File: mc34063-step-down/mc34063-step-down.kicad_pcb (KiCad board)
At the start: 2 copper layers, 82 x 52 mm, 104 parts, among them J1 Vin, J2 Vout, U1 MC34063AD, U2 220uH

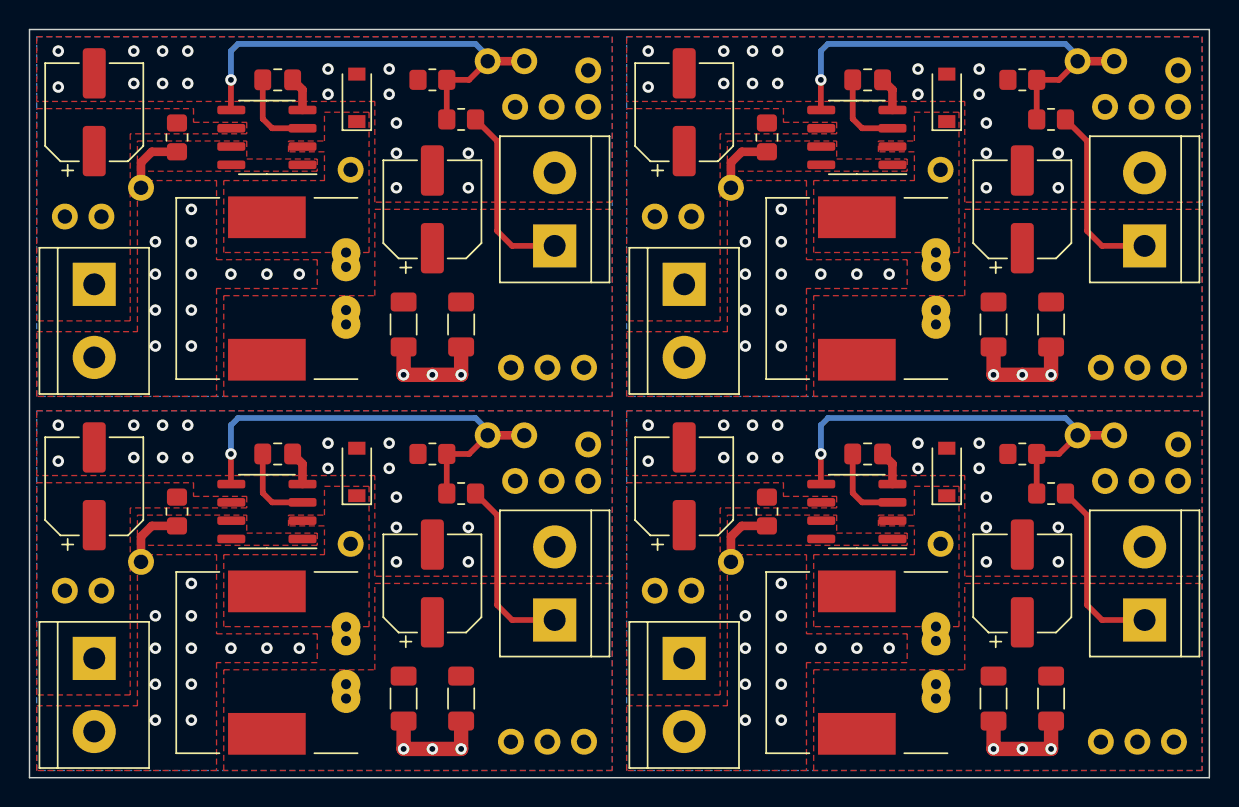
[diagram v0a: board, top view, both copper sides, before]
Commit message: released dev board
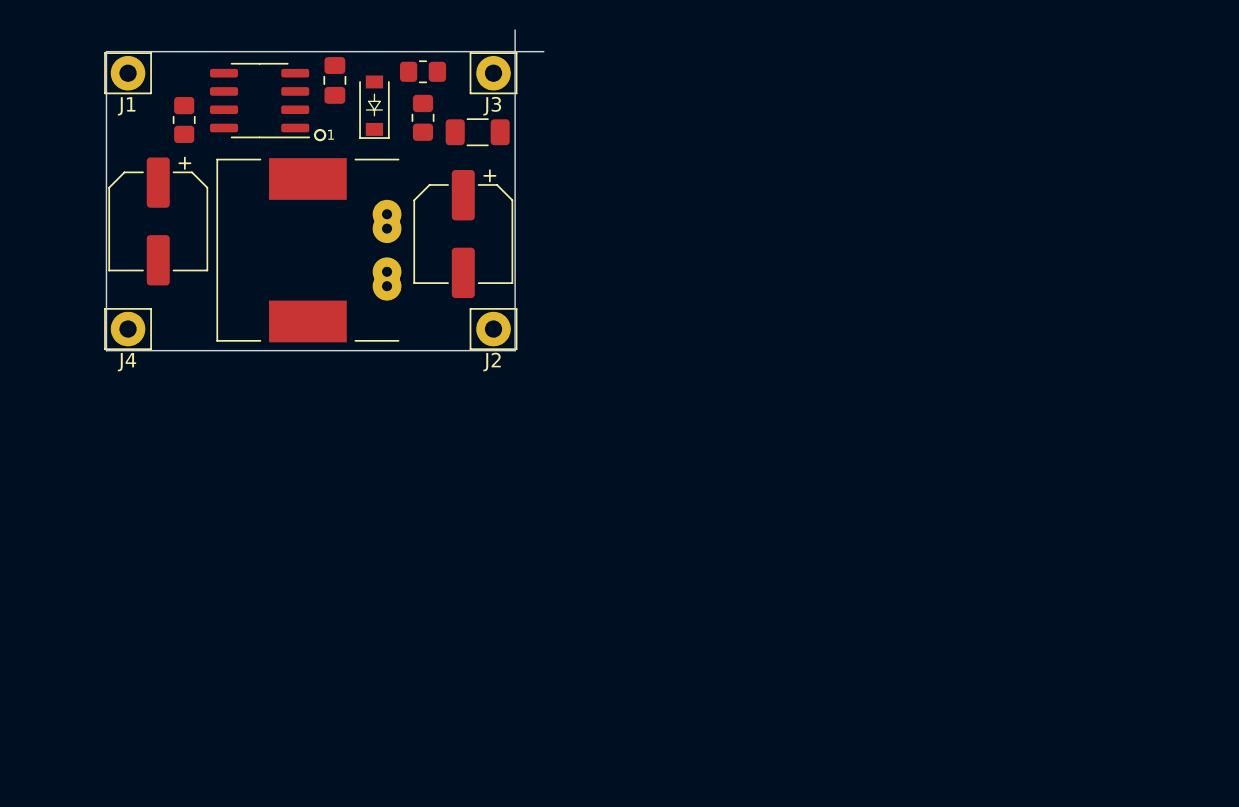
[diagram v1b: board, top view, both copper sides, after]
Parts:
- removed the Ci1 at (116.5, 50.8)
- removed the Ci1 at (116.5, 76.8)
- removed the Ci1 at (75.5, 76.8)
- removed the Co1 at (140.0, 57.5)
- removed the Co1 at (99.0, 83.5)
- removed the Co1 at (140.0, 83.5)
- removed the Co2 at (138.0, 65.5)
- removed the Co2 at (97.0, 91.5)
- removed the Co2 at (138.0, 91.5)
- removed Co3 (x4): 47u/10V, Capacitor_SMD:C_1206_3216Metric_Pad1.33x1.80mm_HandSolder
- removed the Ct1 at (129.2, 74.5)
- removed the Ct1 at (129.2, 48.5)
- removed the Ct1 at (88.2, 74.5)
- removed the D1 at (134.8, 49.8)
- removed the D1 at (93.8, 75.8)
- removed the D1 at (134.8, 75.8)
- removed the J1 at (75.5, 62.7)
- removed the J1 at (116.5, 88.7)
- removed the J1 at (116.5, 62.7)
- removed the J1 at (75.5, 88.7)
- removed the J2 at (107.5, 86.0)
- removed the J2 at (148.5, 60.0)
- removed the J2 at (148.5, 86.0)
- removed the J2 at (107.5, 60.0)
- removed the R1 at (142.0, 77.2)
- removed the R1 at (142.0, 51.2)
- removed the R1 at (101.0, 77.2)
- removed the R2 at (140.0, 74.5)
- removed the R2 at (99.0, 74.5)
- removed the R2 at (140.0, 48.5)
- removed the RSC1 at (81.2, 78.5)
- removed the RSC1 at (122.2, 78.5)
- removed the RSC1 at (122.2, 52.5)
- removed TP1 (x4), TP10 (x4), TP11 (x4), TP12 (x4), TP13 (x4), TP2 (x4), TP3 (x4), TP4 (x4), TP5 (x4), TP6 (x4), TP7 (x4), TP8 (x4), TP9 (x4): TestPoint, TestPoint:TestPoint
- removed the U1 at (87.5, 78.5)
- removed the U1 at (128.5, 52.5)
- removed the U1 at (128.5, 78.5)
- removed the U2 at (128.5, 89.0)
- removed the U2 at (87.5, 89.0)
- removed the U2 at (128.5, 63.0)
- removed the U2 at (87.5, 63.0)
- added J1: M, Connector_Pin:Pin_D1.2mm_L10.2mm_W2.9mm_FlatFork, F.Cu at (77.8, 48.0)
- added J2: M, Connector_Pin:Pin_D1.2mm_L10.2mm_W2.9mm_FlatFork, F.Cu at (103.2, 65.8)
- added J3: M, Connector_Pin:Pin_D1.2mm_L10.2mm_W2.9mm_FlatFork, F.Cu at (103.2, 48.0)
- added J4: M, Connector_Pin:Pin_D1.2mm_L10.2mm_W2.9mm_FlatFork, F.Cu at (77.8, 65.8)
- added U2: 220uH, mc34063-power-inductor:mc34063-power-inductor, F.Cu at (90.3, 60.3)
- moved Co2 14.3 mm to (102.2, 52.1), turned to 0 degrees
- moved Ci1 8.80 mm to (80.0, 58.3), turned to -90 degrees
- moved Ct1 3.97 mm to (92.2, 48.5), turned to 90 degrees
- moved Co1 2.75 mm to (101.2, 59.2), turned to -90 degrees
- moved R1 2.65 mm to (98.3, 51.1), turned to 90 degrees
- moved U1 2.61 mm to (87.0, 49.9)
- moved D1 1.34 mm to (95.0, 50.3)
- moved RSC1 1.31 mm to (81.8, 51.3)
- moved R2 0.86 mm to (98.3, 47.9)
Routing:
- net /Vfeedback: track 126.2 -> 0.00 mm, vias 4 -> 0
- net /Vout: track 51.2 -> 0.00 mm
- net GND: track 42.7 -> 0.00 mm, vias 128 -> 0
- net Net-(Ct1-Pad1): track 23.0 -> 0.00 mm
- net /Sense: track 18.2 -> 0.00 mm
- removed copper zone on F.Cu, net /In
- removed copper zone on F.Cu, net /Sense
- removed copper zone on F.Cu, net /Vout
- removed copper zone on B.Cu, net GND
- removed copper zone on F.Cu, net GND
- removed copper zone on F.Cu, net Net-(D1-Pad1)
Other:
- board size 82 x 52 mm -> 30.4 x 22.3 mm
- board text added: "1"
- board text added: "add pads for pcb TH mounting add silkscreens remove silk from connectors and screw holes"
